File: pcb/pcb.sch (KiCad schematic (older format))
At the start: 1 part, among them U1 NodeMCU1.0(ESP-12E)

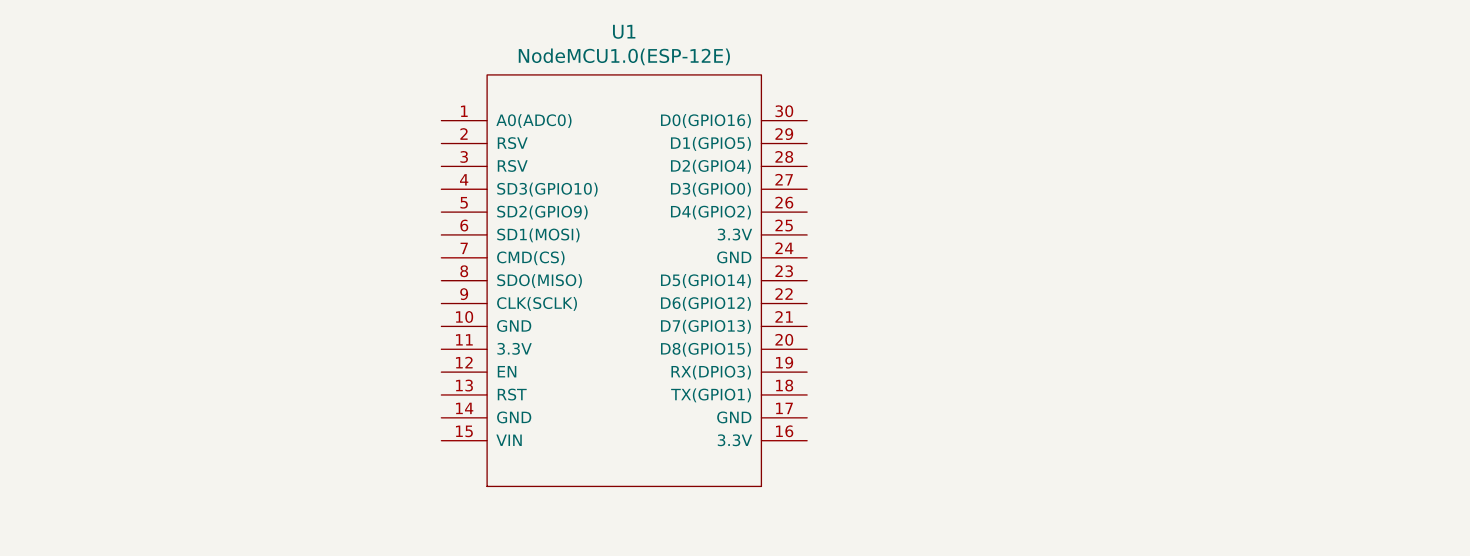
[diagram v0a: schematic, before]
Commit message: First PCB revision complete
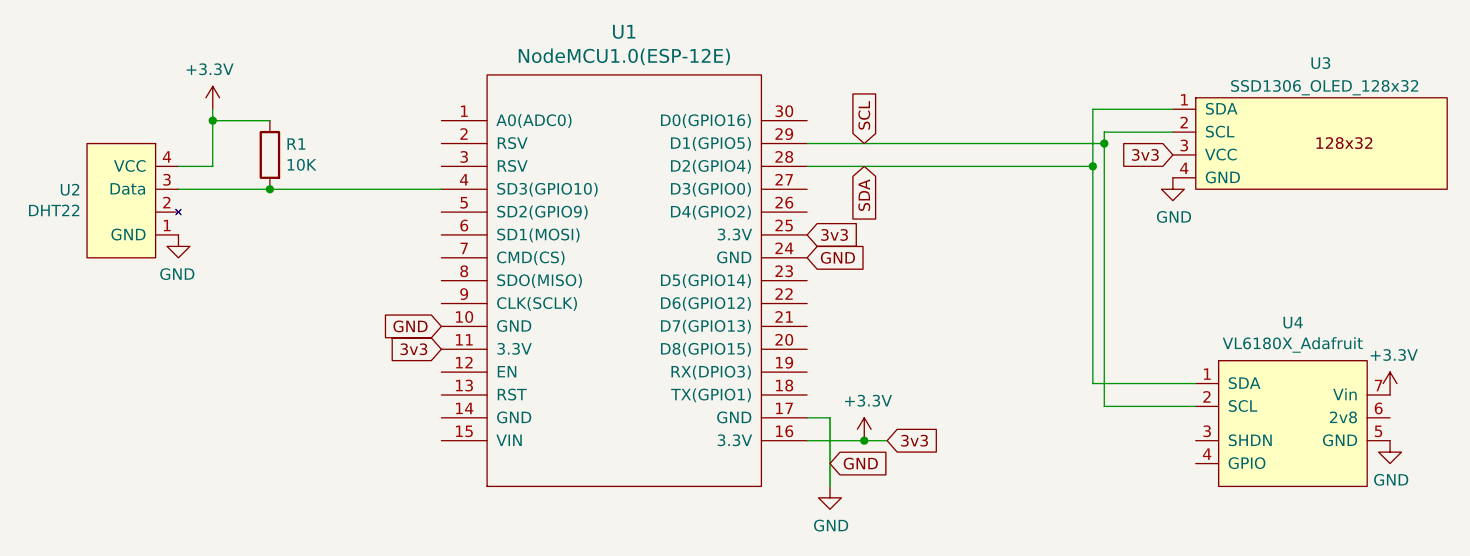
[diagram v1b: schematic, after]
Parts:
- added R1: 10K, Resistor_THT:R_Axial_DIN0204_L3.6mm_D1.6mm_P7.62mm_Horizontal, symbol Device:R
- added U2: DHT22, Connector_PinSocket_2.54mm:PinSocket_1x04_P2.54mm_Horizontal, symbol sensors:DHT22
- added U3: SSD1306_OLED_128x32, personal:SSD1306_OLED_128x32, symbol sensors:SSD1306_OLED_128x32
- added U4: VL6180X_Adafruit, personal:VL6180X_Adafruit, symbol sensors:VL6180X_Adafruit
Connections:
- net GND: now reaches U1.10 (GND)
- net GND: now also U1.17 (GND), U1.24 (GND), U2.1 (GND), U3.4 (GND), U4.5 (GND)
- net +3V3: now reaches U1.11 (3.3V)
- net +3V3: now also U1.16 (3.3V), U1.25 (3.3V), R1.1, U2.4 (VCC), U3.3 (VCC), U4.7 (Vin)
- net SDA: now reaches U1.28 (D2(GPIO4))
- net SDA: now also U3.1 (SDA), U4.1 (SDA)
- net SCL: now reaches U1.29 (D1(GPIO5))
- net SCL: now also U3.2 (SCL), U4.2 (SCL)
- net at U1.4 (SD3(GPIO10)): now also R1.2, U2.3 (Data)
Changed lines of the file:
@@
 EESchema Schematic File Version 4
+LIBS:pcb-cache
 EELAYER 26 0
 EELAYER END
@@
 	1    0    0    -1
 $EndComp
+$Comp
+L sensors:DHT22 U2
+U 1 1 5EB9C5AE
+P 3850 3650
+F 0 "U2" H 4027 3746 50  0000 L CNN
+F 1 "DHT22" H 4027 3655 50  0000 L CNN
+F 2 "Connector_PinSocket_2.54mm:PinSocket_1x04_P2.54mm_Horizontal" H 3700 3750 50  0001 C CNN
+F 3 "" H 3700 3750 50  0001 C CNN
+	1    3850 3650
+	-1   0    0    -1
+$EndComp
+$Comp
+L sensors:SSD1306_OLED_128x32 U3
+U 1 1 5EBADA8A
+P 9050 3400
+F 0 "U3" H 9050 3800 50  0000 L CNN
+F 1 "SSD1306_OLED_128x32" H 8700 3700 50  0000 L CNN
+F 2 "personal:SSD1306_OLED_128x32" H 8550 3750 50  0001 C CNN
+F 3 "" H 8550 3750 50  0001 C CNN
+	1    9050 3400
+	1    0    0    -1
+$EndComp
+$Comp
+L Device:R R1
+U 1 1 5EBADE24
+P 4500 3400
+F 0 "R1" H 4430 3446 50  0000 R CNN
+F 1 "10K" H 4430 3355 50  0000 R CNN
+F 2 "Resistor_THT:R_Axial_DIN0204_L3.6mm_D1.6mm_P7.62mm_Horizontal" V 4430 3400 50  0001 C CNN
+F 3 "~" H 4500 3400 50  0001 C CNN
+	1    4500 3400
+	-1   0    0    -1
+$EndComp
+$Comp
+L power:GND #PWR0101
+U 1 1 5EBADF75
+P 4100 3750
+F 0 "#PWR0101" H 4100 3500 50  0001 C CNN
+F 1 "GND" H 4105 3577 50  0000 C CNN
+F 2 "" H 4100 3750 50  0001 C CNN
+F 3 "" H 4100 3750 50  0001 C CNN
+	1    4100 3750
+	-1   0    0    -1
+$EndComp
+$Comp
+L power:+3.3V #PWR0102
+U 1 1 5EBADFC6
+P 4250 3200
+F 0 "#PWR0102" H 4250 3050 50  0001 C CNN
+F 1 "+3.3V" H 4265 3373 50  0000 C CNN
+F 2 "" H 4250 3200 50  0001 C CNN
+F 3 "" H 4250 3200 50  0001 C CNN
+	1    4250 3200
+	-1   0    0    -1
+$EndComp
+Wire Wire Line
+	4100 3450 4250 3450
+Wire Wire Line
+	4250 3450 4250 3250
+Wire Wire Line
+	4500 3250 4250 3250
+Connection ~ 4250 3250
+Wire Wire Line
+	4250 3250 4250 3200
+Wire Wire Line
+	4100 3550 4500 3550
+Wire Wire Line
+	5250 3550 4500 3550
+Connection ~ 4500 3550
+$Comp
+L power:+3.3V #PWR0103
+U 1 1 5EBAE54C
+P 7100 4650
+F 0 "#PWR0103" H 7100 4500 50  0001 C CNN
+F 1 "+3.3V" H 7115 4823 50  0000 C CNN
+F 2 "" H 7100 4650 50  0001 C CNN
+F 3 "" H 7100 4650 50  0001 C CNN
+	1    7100 4650
+	1    0    0    -1
+$EndComp
+Text GLabel 7100 3450 3    50   Input ~ 0
+SDA
+Text GLabel 7100 3350 1    50   Input ~ 0
+SCL
+$Comp
+L sensors:VL6180X_Adafruit U4
+U 1 1 5EBAEF0A
+P 8950 4600
+F 0 "U4" H 8975 5065 50  0000 C CNN
+F 1 "VL6180X_Adafruit" H 8975 4974 50  0000 C CNN
+F 2 "personal:VL6180X_Adafruit" H 9000 4250 50  0001 C CNN
+F 3 "" H 9000 4250 50  0001 C CNN
+	1    8950 4600
+	1    0    0    -1
+$EndComp
+$Comp
+L power:+3.3V #PWR0104
+U 1 1 5EBAF0BC
+P 9400 4450
+F 0 "#PWR0104" H 9400 4300 50  0001 C CNN
+F 1 "+3.3V" H 9415 4623 50  0000 C CNN
+F 2 "" H 9400 4450 50  0001 C CNN
+F 3 "" H 9400 4450 50  0001 C CNN
+	1    9400 4450
+	1    0    0    -1
+$EndComp
+$Comp
+L power:GND #PWR0105
+U 1 1 5EBAF0F4
+P 9400 4650
+F 0 "#PWR0105" H 9400 4400 50  0001 C CNN
+F 1 "GND" H 9405 4477 50  0000 C CNN
+F 2 "" H 9400 4650 50  0001 C CNN
+F 3 "" H 9400 4650 50  0001 C CNN
+	1    9400 4650
+	1    0    0    -1
+$EndComp
+$Comp
+L power:GND #PWR0106
+U 1 1 5EBAF125
+P 8450 3500
+F 0 "#PWR0106" H 8450 3250 50  0001 C CNN
+F 1 "GND" H 8455 3327 50  0000 C CNN
+F 2 "" H 8450 3500 50  0001 C CNN
+F 3 "" H 8450 3500 50  0001 C CNN
+	1    8450 3500
+	1    0    0    -1
+$EndComp
+Wire Wire Line
+	8450 3200 8100 3200
+Wire Wire Line
+	8100 3200 8100 3450
+Wire Wire Line
+	8100 4400 8550 4400
+Wire Wire Line
+	8450 3300 8150 3300
+Wire Wire Line
+	8150 3300 8150 3350
+Wire Wire Line
+	8150 4500 8550 4500
+Text GLabel 7200 4650 2    50   Input ~ 0
+3v3
+Text GLabel 8450 3400 0    50   Input ~ 0
+3v3
+Wire Wire Line
+	6850 3450 8100 3450
+Connection ~ 8100 3450
+Wire Wire Line
+	8100 3450 8100 4400
+Wire Wire Line
+	6850 3350 8150 3350
+Connection ~ 8150 3350
+Wire Wire Line
+	8150 3350 8150 4500
+Wire Wire Line
+	6850 4650 7100 4650
+Wire Wire Line
+	7100 4650 7200 4650
+Connection ~ 7100 4650
+$Comp
+L power:GND #PWR0107
+U 1 1 5EBAFEB9
+P 6950 4850
+F 0 "#PWR0107" H 6950 4600 50  0001 C CNN
+F 1 "GND" H 6955 4677 50  0000 C CNN
+F 2 "" H 6950 4850 50  0001 C CNN
+F 3 "" H 6950 4850 50  0001 C CNN
+	1    6950 4850
+	1    0    0    -1
+$EndComp
+Wire Wire Line
+	6850 4550 6950 4550
+Text GLabel 6850 3750 2    50   Input ~ 0
+3v3
+Text GLabel 6850 3850 2    50   Input ~ 0
+GND
+Text GLabel 6950 4750 2    50   Input ~ 0
+GND
+Wire Wire Line
+	6950 4550 6950 4850
+Text GLabel 5250 4150 0    50   Input ~ 0
+GND
+Text GLabel 5250 4250 0    50   Input ~ 0
+3v3
 $EndSCHEMATC
